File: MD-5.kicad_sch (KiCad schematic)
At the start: 37 parts

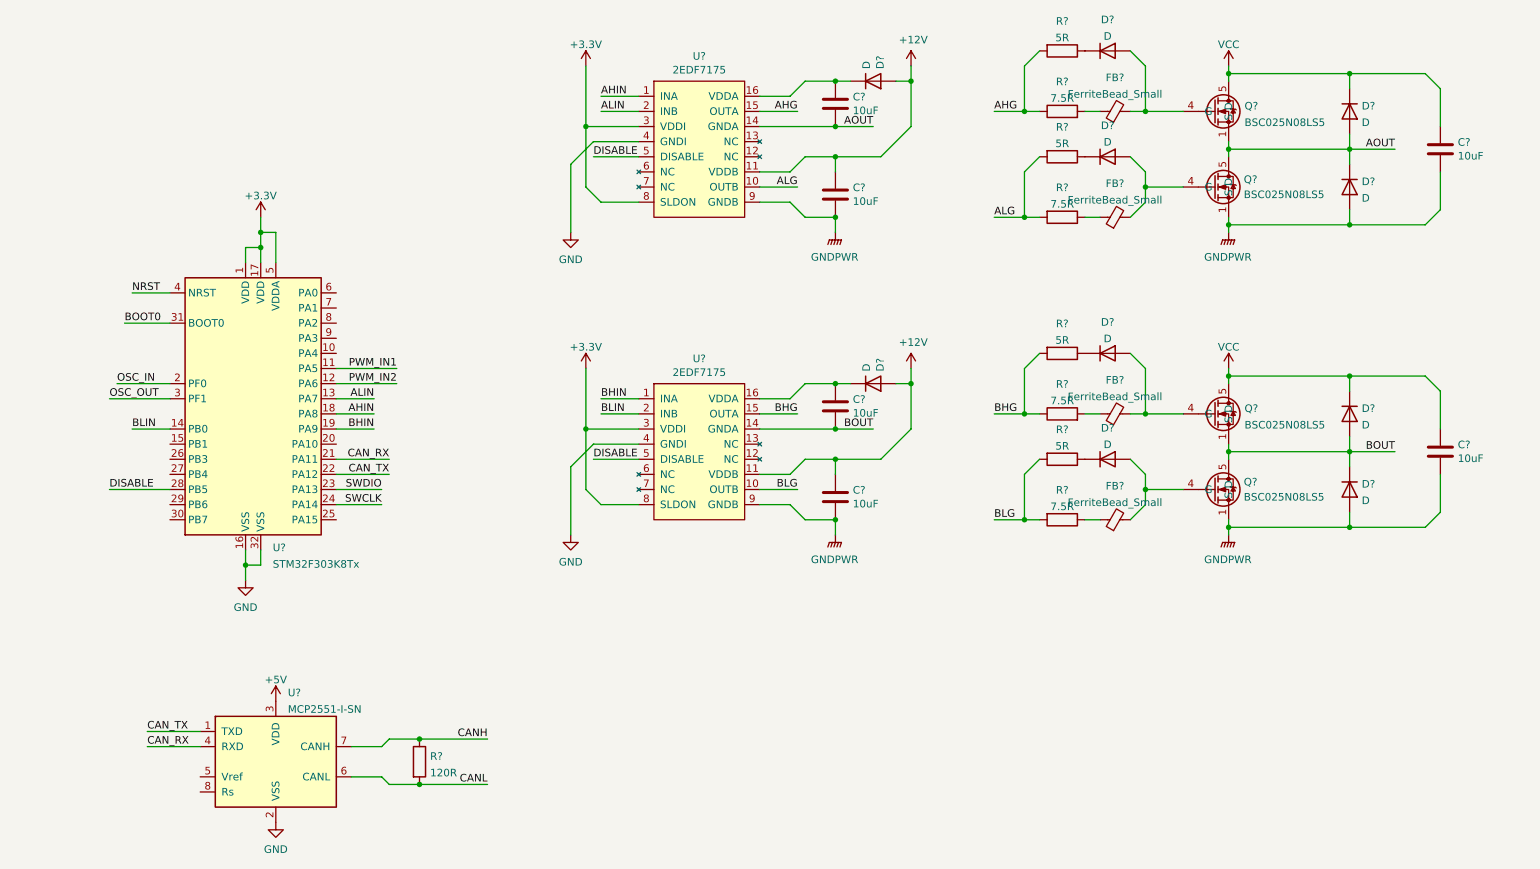
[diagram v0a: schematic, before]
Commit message: mcushuuhen
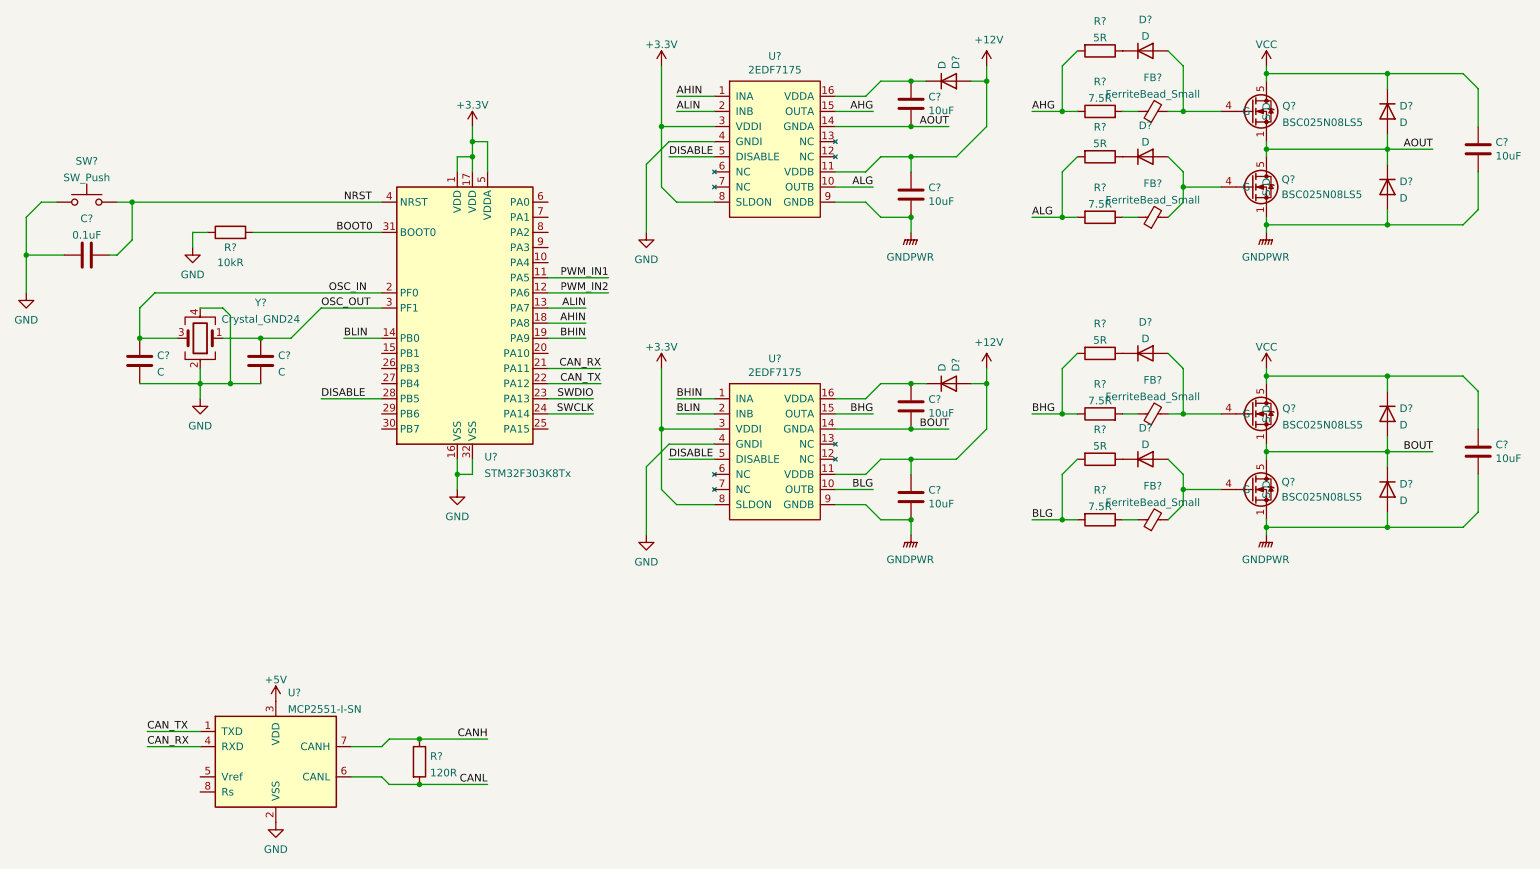
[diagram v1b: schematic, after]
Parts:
- added C? (x2): C, Capacitor_SMD:C_0603_1608Metric, symbol Device:C
- added C?: 0.1uF, Capacitor_SMD:C_0603_1608Metric, symbol Device:C
- added R?: 10kR, Resistor_SMD:R_0603_1608Metric, symbol Device:R
- added SW?: SW_Push, Button_Switch_additional:TVAF06-A020B-R, symbol Switch:SW_Push
- added Y?: Crystal_GND24, Crystal:Crystal_SMD_3225-4Pin_3.2x2.5mm, symbol Device:Crystal_GND24
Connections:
- net BOOT0: now also R?.2
- net GND: now also C?.2, C?.2, C?.2, R?.1, SW?.1, Y?.2, Y?.4
- net NRST: now also C?.1, SW?.2
- net OSC_IN: now also C?.1, Y?.3
- net OSC_OUT: now also C?.1, Y?.1
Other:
- moved on the sheet: C?, D?, FB?, Q?, R?, U?
